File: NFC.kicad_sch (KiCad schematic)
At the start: 24 parts, among them U5 MFRC52202HN1_157, Y1 27.12MHz

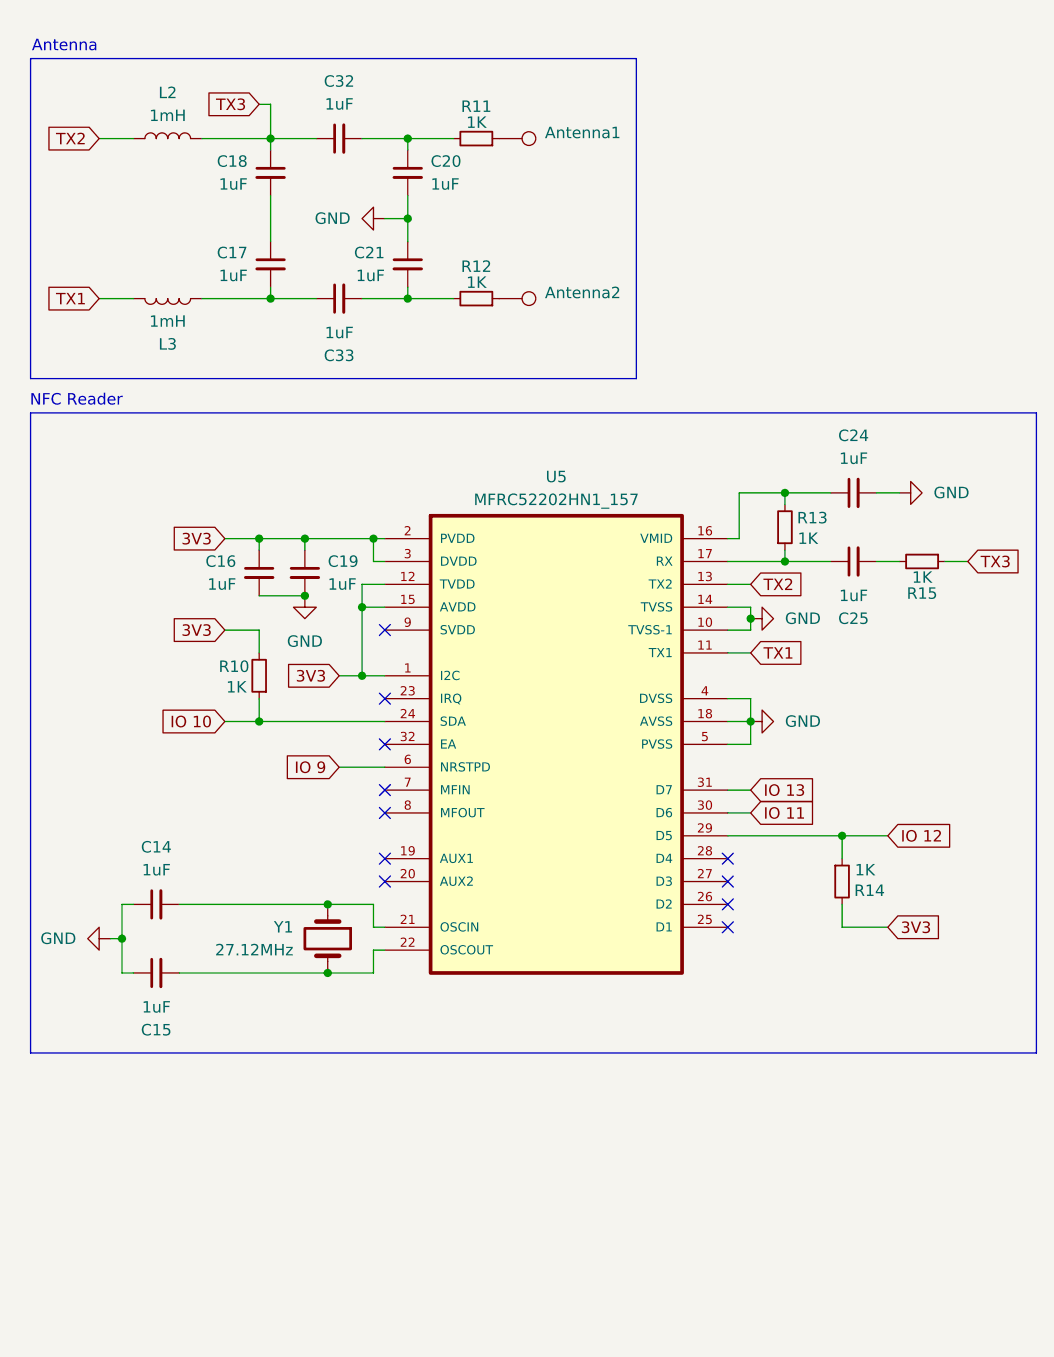
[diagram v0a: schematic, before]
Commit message: Create PCB
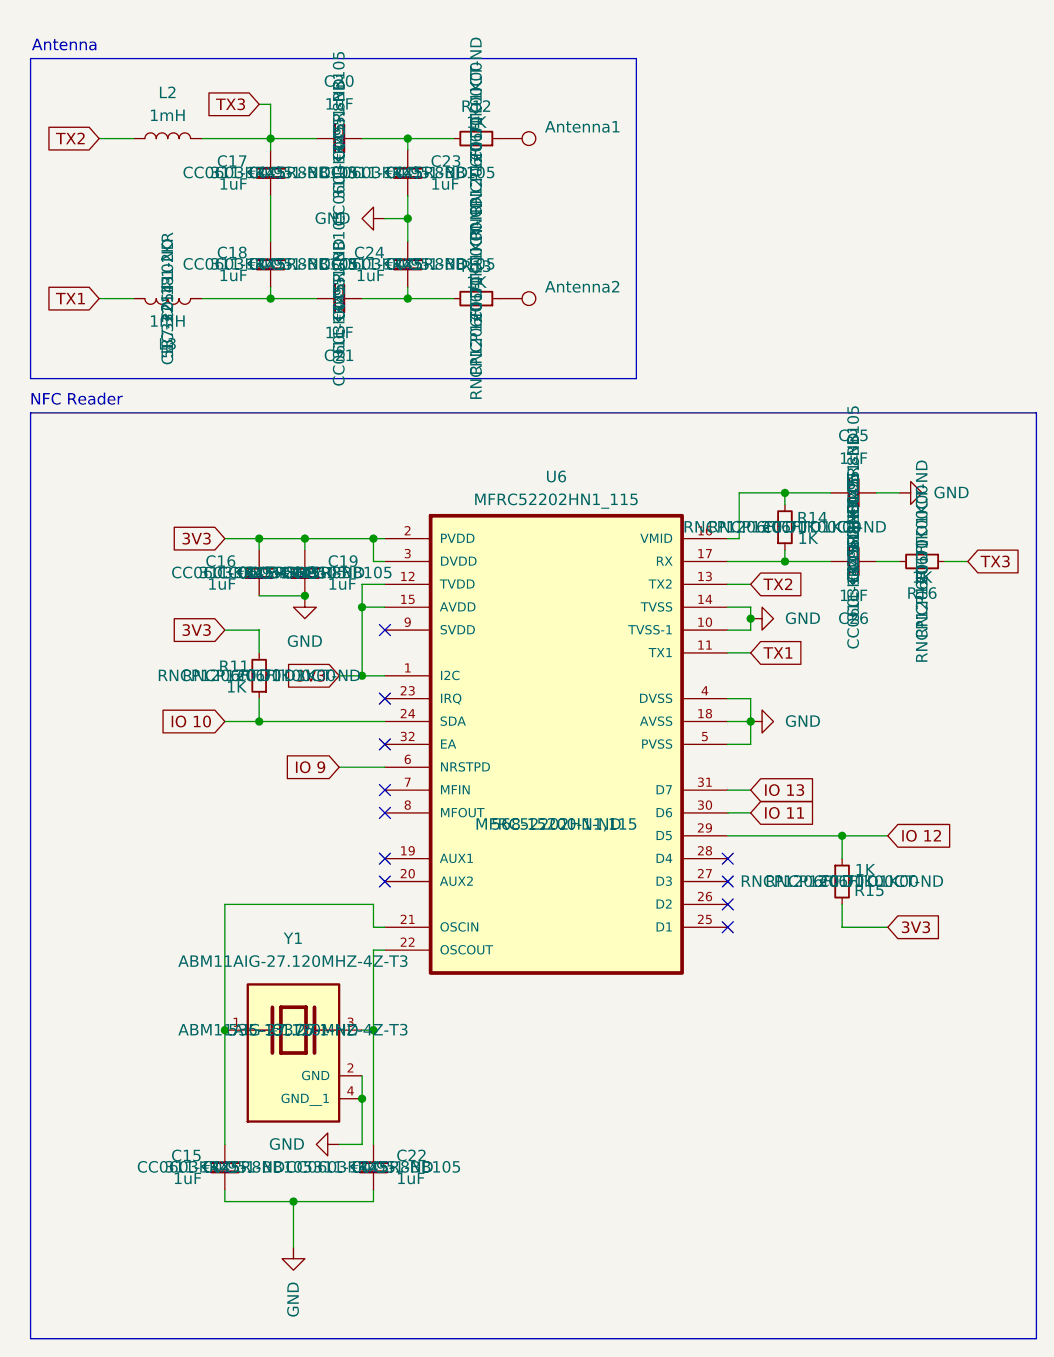
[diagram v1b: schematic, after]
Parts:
- removed C14: 1uF, Capacitor_SMD:C_0603_1608Metric, symbol Device:C_Small
- removed Y1: 27.12MHz, Crystal:Crystal_HC18-U_Vertical, symbol Device:Crystal
- added C22: 1uF, Capacitor_SMD:C_0603_1608Metric, symbol Device:C_Small
- added Y1: ABM11AIG-27.120MHZ-4Z-T3, Footprints:XTAL_ABM11AIG-27.120MHZ-4Z-T3, symbol ABM11AIG-27.120MHZ-4Z-T3:ABM11AIG-27.120MHZ-4Z-T3
- Antenna1, Antenna2: footprint TestPoint:TestPoint_Pad_D4.0mm -> TestPoint:TestPoint_Pad_D2.0mm
- C15, C16, C19: DigiKey_Part_Number (none) -> 311-1445-1-ND; Manufacturer_Part_Number (none) -> CC0603KRX5R8BB105; Price (none) -> €0.95
- C17: renamed from C18; DigiKey_Part_Number (none) -> 311-1445-1-ND; Manufacturer_Part_Number (none) -> CC0603KRX5R8BB105; Price (none) -> €0.95
- C18: renamed from C17; DigiKey_Part_Number (none) -> 311-1445-1-ND; Manufacturer_Part_Number (none) -> CC0603KRX5R8BB105; Price (none) -> €0.95
- C20: renamed from C32; DigiKey_Part_Number (none) -> 311-1445-1-ND; Manufacturer_Part_Number (none) -> CC0603KRX5R8BB105; Price (none) -> €0.95
- C21: renamed from C33; DigiKey_Part_Number (none) -> 311-1445-1-ND; Manufacturer_Part_Number (none) -> CC0603KRX5R8BB105; Price (none) -> €0.95
- C23: renamed from C20; DigiKey_Part_Number (none) -> 311-1445-1-ND; Manufacturer_Part_Number (none) -> CC0603KRX5R8BB105; Price (none) -> €0.95
- C24: renamed from C21; DigiKey_Part_Number (none) -> 311-1445-1-ND; Manufacturer_Part_Number (none) -> CC0603KRX5R8BB105; Price (none) -> €0.95
- C25: renamed from C24; DigiKey_Part_Number (none) -> 311-1445-1-ND; Manufacturer_Part_Number (none) -> CC0603KRX5R8BB105; Price (none) -> €0.95
- C26: renamed from C25; DigiKey_Part_Number (none) -> 311-1445-1-ND; Manufacturer_Part_Number (none) -> CC0603KRX5R8BB105; Price (none) -> €0.95
- L2, L3: footprint Inductor_SMD:L_0603_1608Metric -> Inductor_SMD:L_1210_3225Metric; DigiKey_Part_Number (none) -> 587-3214-1-ND; Manufacturer_Part_Number (none) -> CBC3225T102KR; Price (none) -> €0.18
- R11: renamed from R10; footprint Resistor_SMD:R_0603_1608Metric -> Resistor_SMD:R_1206_3216Metric; DigiKey_Part_Number (none) -> RNCP1206FTD1K00CT-ND; Manufacturer_Part_Number (none) -> RNCP1206FTD1K00; Price (none) -> €0.70
- R12: renamed from R11; footprint Resistor_SMD:R_0603_1608Metric -> Resistor_SMD:R_1206_3216Metric; DigiKey_Part_Number (none) -> RNCP1206FTD1K00CT-ND; Manufacturer_Part_Number (none) -> RNCP1206FTD1K00; Price (none) -> €0.70
- R13: renamed from R12; footprint Resistor_SMD:R_0603_1608Metric -> Resistor_SMD:R_1206_3216Metric; DigiKey_Part_Number (none) -> RNCP1206FTD1K00CT-ND; Manufacturer_Part_Number (none) -> RNCP1206FTD1K00; Price (none) -> €0.70
- R14: renamed from R13; footprint Resistor_SMD:R_0603_1608Metric -> Resistor_SMD:R_1206_3216Metric; DigiKey_Part_Number (none) -> RNCP1206FTD1K00CT-ND; Manufacturer_Part_Number (none) -> RNCP1206FTD1K00; Price (none) -> €0.70
- R15: renamed from R14; footprint Resistor_SMD:R_0603_1608Metric -> Resistor_SMD:R_1206_3216Metric; DigiKey_Part_Number (none) -> RNCP1206FTD1K00CT-ND; Manufacturer_Part_Number (none) -> RNCP1206FTD1K00; Price (none) -> €0.70
- R16: renamed from R15; footprint Resistor_SMD:R_0603_1608Metric -> Resistor_SMD:R_1206_3216Metric; DigiKey_Part_Number (none) -> RNCP1206FTD1K00CT-ND; Manufacturer_Part_Number (none) -> RNCP1206FTD1K00; Price (none) -> €0.70
- U6: renamed from U5; value MFRC52202HN1_157 -> MFRC52202HN1_115; footprint Footprints:IC_PCAL9722HNMP -> Package_DFN_QFN:HVQFN-32-1EP_5x5mm_P0.5mm_EP3.1x3.1mm; Availability In Stock -> (none); Check_prices https://www.snapeda.com/parts/MFRC52202HN1,157/NXP+Semicond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 -> (none); Description_1 RFID Reader IC 13.56MHz ISO 14443, MIFARE I2C, SPI, UART 2.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 -> (none); DigiKey_Part_Number (none) -> 568-15200-1-ND; MF NXP USA -> (none); MP MFRC52202HN1,157 -> (none); Manufacturer NXP USA -> (none); Manufacturer_Part_Number (none) -> MFRC52202HN1,115; Package VFQFN-32 NXP Semiconductors -> (none); Price None -> €7.54; SnapEDA_Link https://www.snapeda.com/parts/MFRC52202HN1,157/NXP+Semicond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 -> (none)
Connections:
- net GND: now also C15.2, C22.2, Y1.2 (GND), Y1.4 (GND__1); no longer C15.1
- net at U6.21 (OSCIN): now also C15.1, Y1.1
- net at U6.22 (OSCOUT): now also C22.1, Y1.3; no longer C15.2
